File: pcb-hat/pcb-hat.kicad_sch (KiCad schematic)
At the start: 17 parts, among them U1 INA219AxD, U3 AOZ6605PI-1

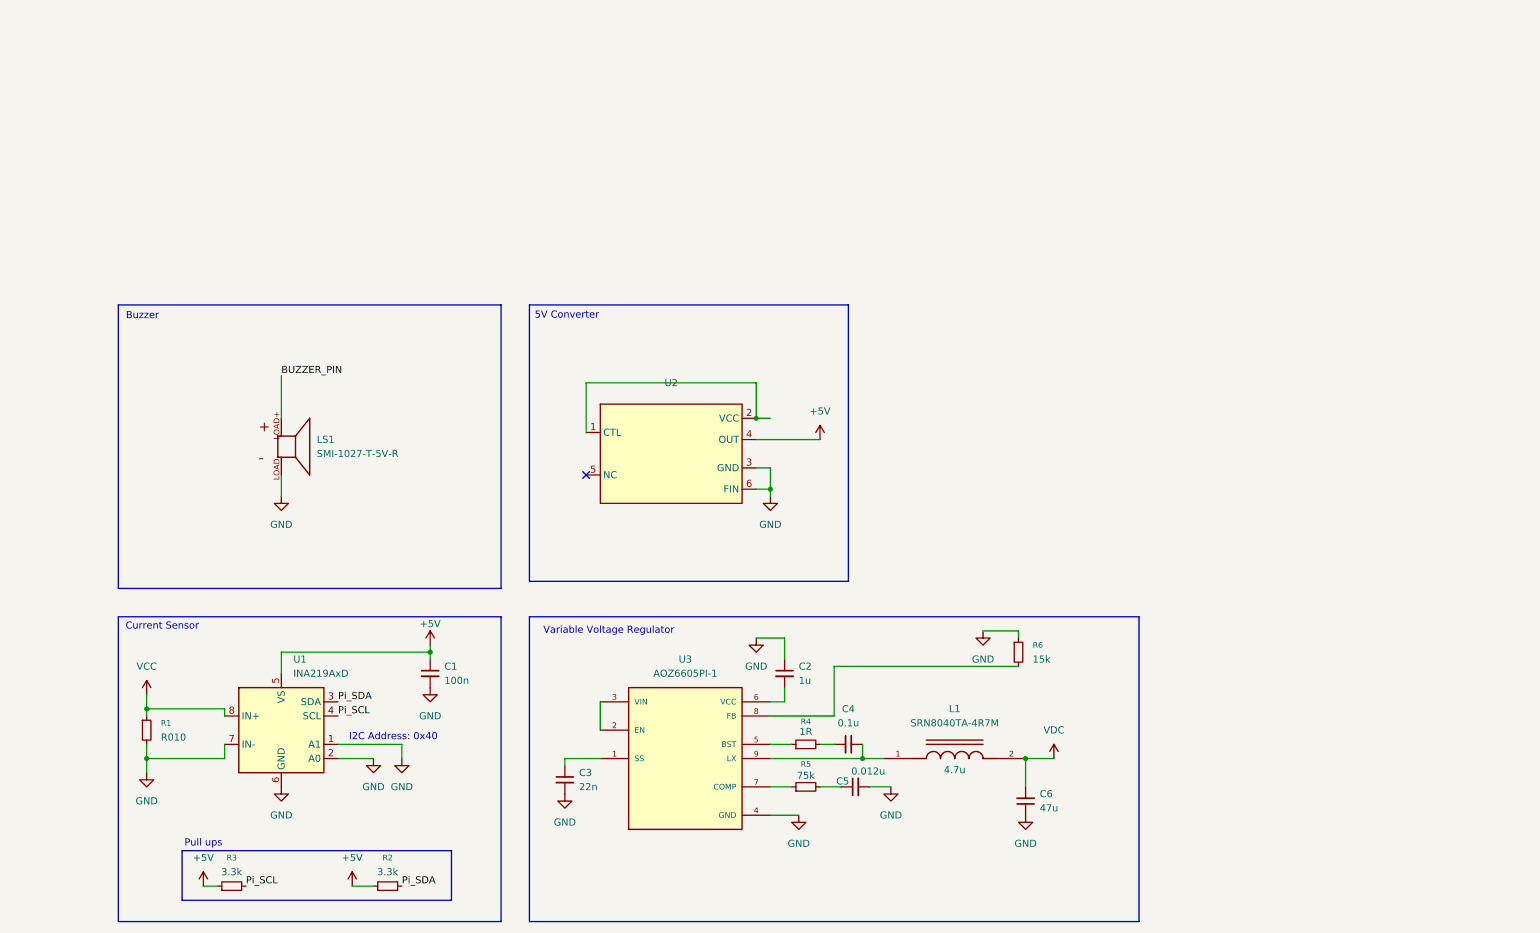
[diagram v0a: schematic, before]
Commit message: Rearrange stuff
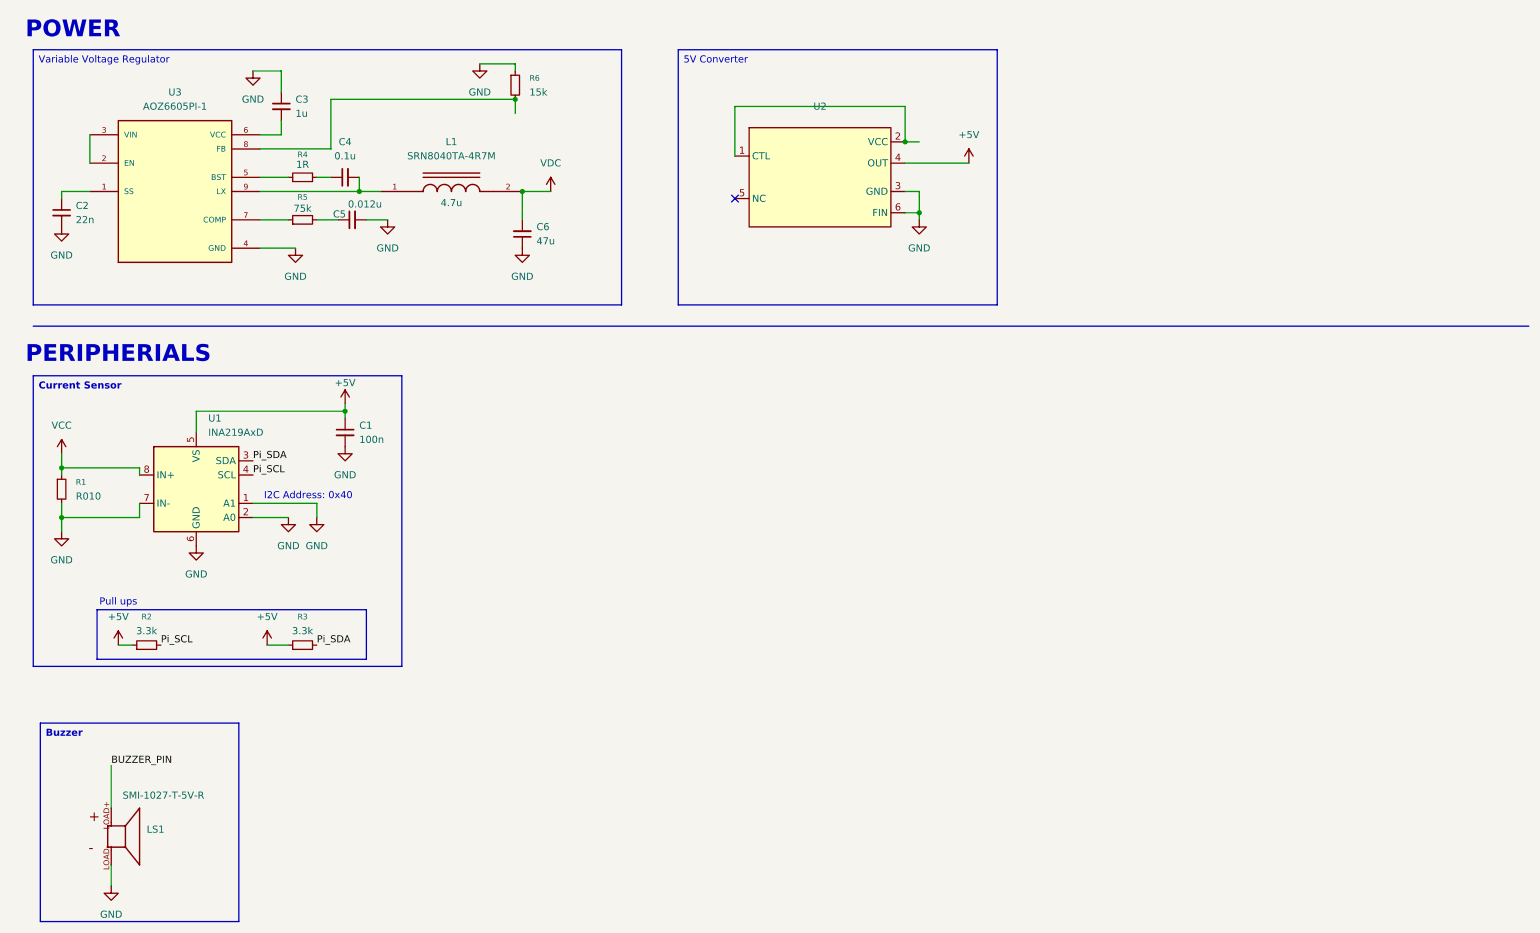
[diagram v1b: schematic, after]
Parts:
- renumbered C3 to C2, C2 to C3, R3 to R2, R2 to R3
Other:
- note added: "PERIPHERIALS"
- note added: "POWER"
- note removed: "Buzzer"
- note removed: "Current Sensor"
- note removed: "Variable Voltage Regulator"
- title: (none) -> Pi Hat
- moved on the sheet: C1, C2, C3, C4, C5, C6, L1, LS1, R1, R2, R3, R4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
